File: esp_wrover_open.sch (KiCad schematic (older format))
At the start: 44 parts, among them J1 USB_B_Micro, J2 Conn_02x13_Counter_Clockwise, J3 Barrel_Jack_Switch, J4 CAN_out, J5 Conn_02x03_Counter_Clockwise, J6 Conn_02x03_Counter_Clockwise, J7 Conn_02x03_Counter_Clockwise, J8 USB_C_Receptacle_USB2.0, Q3 Q_NPN_BCE, Q4 Q_NPN_BCE, SW1 reset, SW2 boot, U1 ESP32-WROVER-B_(16MB), U2 CP2102N, U3 AMS1117-3.3, U4 SN65HVD230, U5 LM1084-5.0

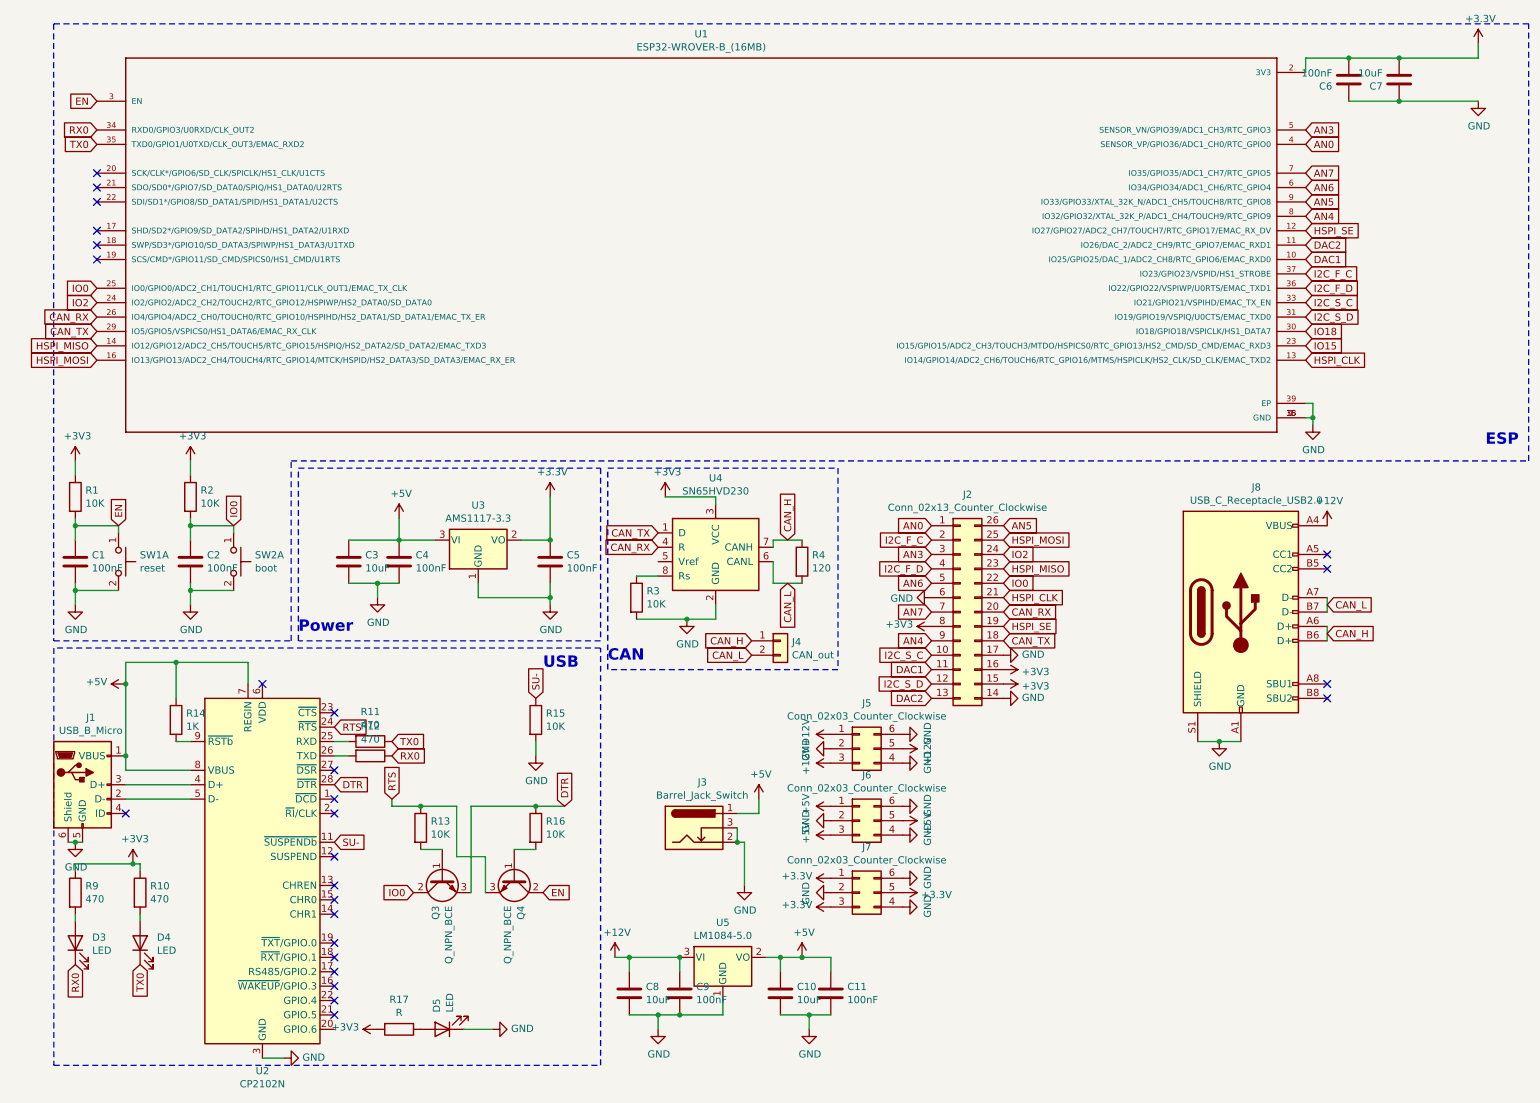
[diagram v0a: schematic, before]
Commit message: update
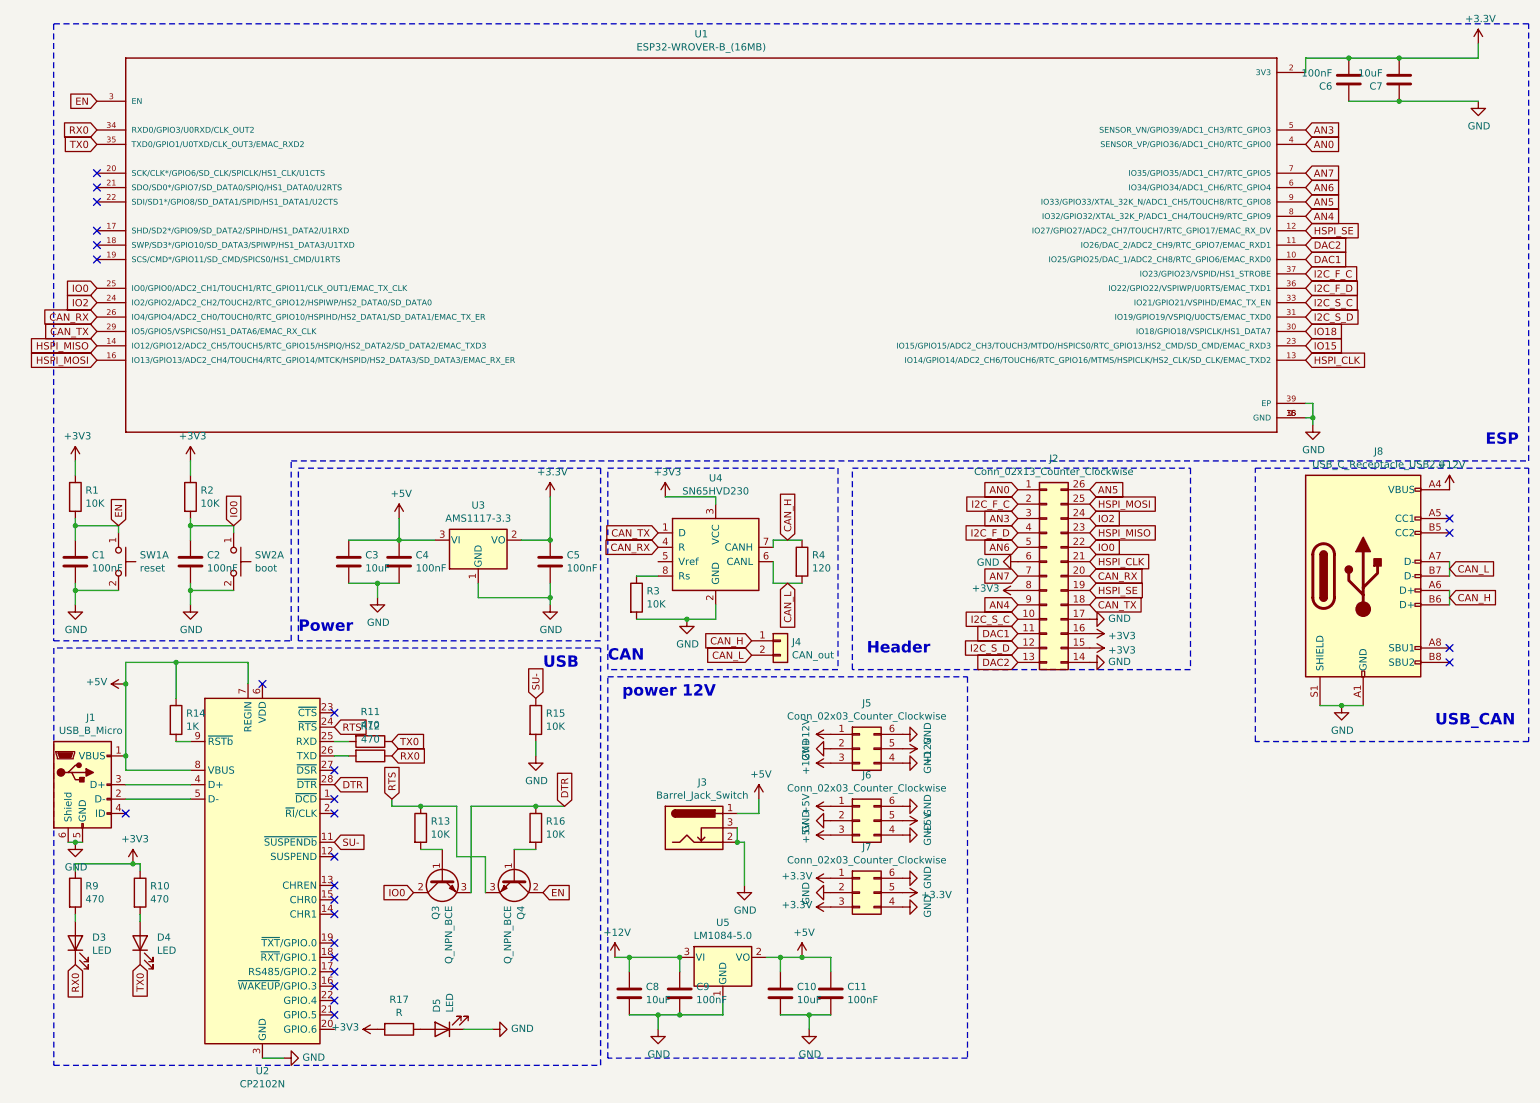
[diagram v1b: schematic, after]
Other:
- note added: "Header"
- note added: "USB_CAN"
- note added: "power 12V"
- moved on the sheet: J2, J8
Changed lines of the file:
@@
 	1    0    0    -1
 $EndComp
-Text GLabel 6600 4000 0    50   Input ~ 0
+Text GLabel 7200 3750 0    50   Input ~ 0
 AN0
 $Comp
 L Connector_Generic:Conn_02x13_Counter_Clockwise J2
 U 1 1 5F00C228
-P 6800 4600
-F 0 "J2" H 6850 5417 50  0000 C CNN
-F 1 "Conn_02x13_Counter_Clockwise" H 6850 5326 50  0000 C CNN
-F 2 "Connector_PinHeader_2.54mm:PinHeader_2x13_P2.54mm_Vertical" H 6800 4600 50  0001 C CNN
-F 3 "~" H 6800 4600 50  0001 C CNN
-	1    6800 4600
-	1    0    0    -1
-$EndComp
-Text GLabel 6600 4200 0    50   Input ~ 0
+P 7400 4350
+F 0 "J2" H 7450 5167 50  0000 C CNN
+F 1 "Conn_02x13_Counter_Clockwise" H 7450 5076 50  0000 C CNN
+F 2 "Connector_PinHeader_2.54mm:PinHeader_2x13_P2.54mm_Vertical" H 7400 4350 50  0001 C CNN
+F 3 "~" H 7400 4350 50  0001 C CNN
+	1    7400 4350
+	1    0    0    -1
+$EndComp
+Text GLabel 7200 3950 0    50   Input ~ 0
 AN3
-Text GLabel 6600 4400 0    50   Input ~ 0
+Text GLabel 7200 4150 0    50   Input ~ 0
 AN6
-Text GLabel 6600 4600 0    50   Input ~ 0
+Text GLabel 7200 4350 0    50   Input ~ 0
 AN7
-Text GLabel 6600 4800 0    50   Input ~ 0
+Text GLabel 7200 4550 0    50   Input ~ 0
 AN4
-Text GLabel 6600 5000 0    50   Input ~ 0
+Text GLabel 7200 4750 0    50   Input ~ 0
 DAC1
-Text GLabel 6600 5200 0    50   Input ~ 0
+Text GLabel 7200 4950 0    50   Input ~ 0
 DAC2
-Text GLabel 7100 4700 2    50   Input ~ 0
+Text GLabel 7700 4450 2    50   Input ~ 0
 HSPI_SE
-Text GLabel 7100 4500 2    50   Input ~ 0
+Text GLabel 7700 4250 2    50   Input ~ 0
 HSPI_CLK
-Text GLabel 7100 4300 2    50   Input ~ 0
+Text GLabel 7700 4050 2    50   Input ~ 0
 HSPI_MISO
-Text GLabel 7100 4100 2    50   Input ~ 0
+Text GLabel 7700 3850 2    50   Input ~ 0
 HSPI_MOSI
-Text GLabel 6600 4100 0    50   Input ~ 0
+Text GLabel 7200 3850 0    50   Input ~ 0
 I2C_F_C
-Text GLabel 6600 4300 0    50   Input ~ 0
+Text GLabel 7200 4050 0    50   Input ~ 0
 I2C_F_D
 $Comp
 L power:+3V3 #PWR0114
 U 1 1 5F039EA4
-P 7100 5100
-F 0 "#PWR0114" H 7100 4950 50  0001 C CNN
-F 1 "+3V3" V 7115 5228 50  0000 L CNN
-F 2 "" H 7100 5100 50  0001 C CNN
-F 3 "" H 7100 5100 50  0001 C CNN
-	1    7100 5100
+P 7700 4850
+F 0 "#PWR0114" H 7700 4700 50  0001 C CNN
+F 1 "+3V3" V 7715 4978 50  0000 L CNN
+F 2 "" H 7700 4850 50  0001 C CNN
+F 3 "" H 7700 4850 50  0001 C CNN
+	1    7700 4850
 	0    1    1    0
 $EndComp
@@
 L power:GND #PWR0115
 U 1 1 5F0397EB
-P 7100 4900
-F 0 "#PWR0115" H 7100 4650 50  0001 C CNN
-F 1 "GND" V 7105 4772 50  0000 R CNN
-F 2 "" H 7100 4900 50  0001 C CNN
-F 3 "" H 7100 4900 50  0001 C CNN
-	1    7100 4900
+P 7700 4650
+F 0 "#PWR0115" H 7700 4400 50  0001 C CNN
+F 1 "GND" V 7705 4522 50  0000 R CNN
+F 2 "" H 7700 4650 50  0001 C CNN
+F 3 "" H 7700 4650 50  0001 C CNN
+	1    7700 4650
 	0    -1   -1   0
 $EndComp
@@
 L power:+3V3 #PWR0116
 U 1 1 5F0462B8
-P 6600 4700
-F 0 "#PWR0116" H 6600 4550 50  0001 C CNN
-F 1 "+3V3" V 6615 4828 50  0000 L CNN
-F 2 "" H 6600 4700 50  0001 C CNN
-F 3 "" H 6600 4700 50  0001 C CNN
-	1    6600 4700
+P 7200 4450
+F 0 "#PWR0116" H 7200 4300 50  0001 C CNN
+F 1 "+3V3" V 7215 4578 50  0000 L CNN
+F 2 "" H 7200 4450 50  0001 C CNN
+F 3 "" H 7200 4450 50  0001 C CNN
+	1    7200 4450
 	0    -1   -1   0
 $EndComp
@@
 L power:GND #PWR0117
 U 1 1 5F04926E
-P 6600 4500
-F 0 "#PWR0117" H 6600 4250 50  0001 C CNN
-F 1 "GND" V 6605 4372 50  0000 R CNN
-F 2 "" H 6600 4500 50  0001 C CNN
-F 3 "" H 6600 4500 50  0001 C CNN
-	1    6600 4500
-	0    1    1    0
-$EndComp
-Text GLabel 6600 4900 0    50   Input ~ 0
+P 7200 4250
+F 0 "#PWR0117" H 7200 4000 50  0001 C CNN
+F 1 "GND" V 7205 4122 50  0000 R CNN
+F 2 "" H 7200 4250 50  0001 C CNN
+F 3 "" H 7200 4250 50  0001 C CNN
+	1    7200 4250
+	0    1    1    0
+$EndComp
+Text GLabel 7200 4650 0    50   Input ~ 0
 I2C_S_C
-Text GLabel 6600 5100 0    50   Input ~ 0
+Text GLabel 7200 4850 0    50   Input ~ 0
 I2C_S_D
 $Comp
 L power:+3V3 #PWR0118
 U 1 1 5F05020F
-P 7100 5000
-F 0 "#PWR0118" H 7100 4850 50  0001 C CNN
-F 1 "+3V3" V 7115 5128 50  0000 L CNN
-F 2 "" H 7100 5000 50  0001 C CNN
-F 3 "" H 7100 5000 50  0001 C CNN
-	1    7100 5000
+P 7700 4750
+F 0 "#PWR0118" H 7700 4600 50  0001 C CNN
+F 1 "+3V3" V 7715 4878 50  0000 L CNN
+F 2 "" H 7700 4750 50  0001 C CNN
+F 3 "" H 7700 4750 50  0001 C CNN
+	1    7700 4750
 	0    1    1    0
 $EndComp
@@
 L power:GND #PWR0119
 U 1 1 5F050215
-P 7100 5200
-F 0 "#PWR0119" H 7100 4950 50  0001 C CNN
-F 1 "GND" V 7105 5072 50  0000 R CNN
-F 2 "" H 7100 5200 50  0001 C CNN
-F 3 "" H 7100 5200 50  0001 C CNN
-	1    7100 5200
-	0    -1   -1   0
-$EndComp
-Text GLabel 7100 4800 2    50   Input ~ 0
+P 7700 4950
+F 0 "#PWR0119" H 7700 4700 50  0001 C CNN
+F 1 "GND" V 7705 4822 50  0000 R CNN
+F 2 "" H 7700 4950 50  0001 C CNN
+F 3 "" H 7700 4950 50  0001 C CNN
+	1    7700 4950
+	0    -1   -1   0
+$EndComp
+Text GLabel 7700 4550 2    50   Input ~ 0
 CAN_TX
-Text GLabel 7100 4600 2    50   Input ~ 0
+Text GLabel 7700 4350 2    50   Input ~ 0
 CAN_RX
-Text GLabel 7100 4400 2    50   Input ~ 0
+Text GLabel 7700 4150 2    50   Input ~ 0
 IO0
-Text GLabel 7100 4200 2    50   Input ~ 0
+Text GLabel 7700 3950 2    50   Input ~ 0
 IO2
 $Comp
@@
 L Connector:USB_C_Receptacle_USB2.0 J8
 U 1 1 5EF61382
-P 8750 4600
-F 0 "J8" H 8857 5467 50  0000 C CNN
-F 1 "USB_C_Receptacle_USB2.0" H 8857 5376 50  0000 C CNN
-F 2 "Connector_USB:USB_C_Receptacle_HRO_TYPE-C-31-M-12" H 8900 4600 50  0001 C CNN
-F 3 "https://www.usb.org/sites/default/files/documents/usb_type-c.zip" H 8900 4600 50  0001 C CNN
-	1    8750 4600
-	1    0    0    -1
-$EndComp
-Wire Wire Line
-	9350 4500 9350 4600
-Wire Wire Line
-	9350 4700 9350 4800
-Wire Wire Line
-	8450 5500 8600 5500
+P 9600 4350
+F 0 "J8" H 9707 5217 50  0000 C CNN
+F 1 "USB_C_Receptacle_USB2.0" H 9707 5126 50  0000 C CNN
+F 2 "Connector_USB:USB_C_Receptacle_HRO_TYPE-C-31-M-12" H 9750 4350 50  0001 C CNN
+F 3 "https://www.usb.org/sites/default/files/documents/usb_type-c.zip" H 9750 4350 50  0001 C CNN
+	1    9600 4350
+	1    0    0    -1
+$EndComp
+Wire Wire Line
+	10200 4250 10200 4350
+Wire Wire Line
+	10200 4450 10200 4550
+Wire Wire Line
+	9300 5250 9450 5250
 $Comp
 L power:GND #PWR0127
 U 1 1 5EF6C465
-P 8600 5500
-F 0 "#PWR0127" H 8600 5250 50  0001 C CNN
-F 1 "GND" H 8605 5327 50  0000 C CNN
-F 2 "" H 8600 5500 50  0001 C CNN
-F 3 "" H 8600 5500 50  0001 C CNN
-	1    8600 5500
-	1    0    0    -1
-$EndComp
-Connection ~ 8600 5500
-Wire Wire Line
-	8600 5500 8750 5500
+P 9450 5250
+F 0 "#PWR0127" H 9450 5000 50  0001 C CNN
+F 1 "GND" H 9455 5077 50  0000 C CNN
+F 2 "" H 9450 5250 50  0001 C CNN
+F 3 "" H 9450 5250 50  0001 C CNN
+	1    9450 5250
+	1    0    0    -1
+$EndComp
+Connection ~ 9450 5250
+Wire Wire Line
+	9450 5250 9600 5250
 $Comp
 L power:+12V #PWR0131
 U 1 1 5EF6FE81
-P 9350 4000
-F 0 "#PWR0131" H 9350 3850 50  0001 C CNN
-F 1 "+12V" H 9365 4173 50  0000 C CNN
-F 2 "" H 9350 4000 50  0001 C CNN
-F 3 "" H 9350 4000 50  0001 C CNN
-	1    9350 4000
-	1    0    0    -1
-$EndComp
-Text GLabel 9350 4750 2    50   Input ~ 0
+P 10200 3750
+F 0 "#PWR0131" H 10200 3600 50  0001 C CNN
+F 1 "+12V" H 10215 3923 50  0000 C CNN
+F 2 "" H 10200 3750 50  0001 C CNN
+F 3 "" H 10200 3750 50  0001 C CNN
+	1    10200 3750
+	1    0    0    -1
+$EndComp
+Text GLabel 10200 4500 2    50   Input ~ 0
 CAN_H
-Text GLabel 9350 4550 2    50   Input ~ 0
+Text GLabel 10200 4300 2    50   Input ~ 0
 CAN_L
-NoConn ~ 9350 4200
-NoConn ~ 9350 4300
-NoConn ~ 9350 5100
-NoConn ~ 9350 5200
+NoConn ~ 10200 3950
+NoConn ~ 10200 4050
+NoConn ~ 10200 4850
+NoConn ~ 10200 4950
 $Comp
 L Regulator_Linear:LM1084-5.0 U5
@@
 	0    -1   -1   0
 $EndComp
-Text GLabel 7100 4000 2    50   Input ~ 0
+Text GLabel 7700 3750 2    50   Input ~ 0
 AN5
+Wire Notes Line
+	6050 3600 8400 3600
+Wire Notes Line
+	8400 3600 8400 5000
+Wire Notes Line
+	8400 5000 6050 5000
+Wire Notes Line
+	6050 5000 6050 3600
+Wire Notes Line
+	8850 3600 10750 3600
+Wire Notes Line
+	10750 3600 10750 5500
+Wire Notes Line
+	10750 5500 8850 5500
+Wire Notes Line
+	8850 5500 8850 3600
+Wire Notes Line
+	4350 5050 6850 5050
+Wire Notes Line
+	6850 5050 6850 7700
+Wire Notes Line
+	6850 7700 4350 7700
+Wire Notes Line
+	4350 7700 4350 5050
+Text Notes 4450 5200 0    79   ~ 16
+power 12V
+Text Notes 6150 4900 0    79   ~ 16
+Header
+Text Notes 10100 5400 0    79   ~ 16
+USB_CAN
 $EndSCHEMATC
